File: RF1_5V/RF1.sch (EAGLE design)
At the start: 13 parts, among them J1 5v, Q1 16mhz, U1 ATMEGA328P_PDIP

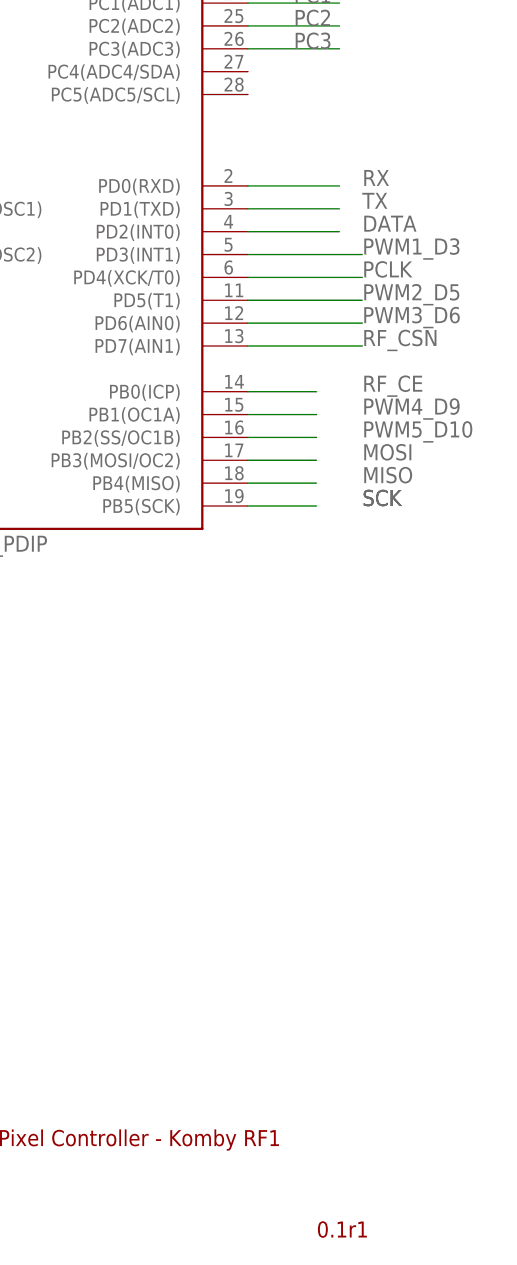
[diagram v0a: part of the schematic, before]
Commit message: Updated with 2014 designs for both RF1_12v and RF1 5v
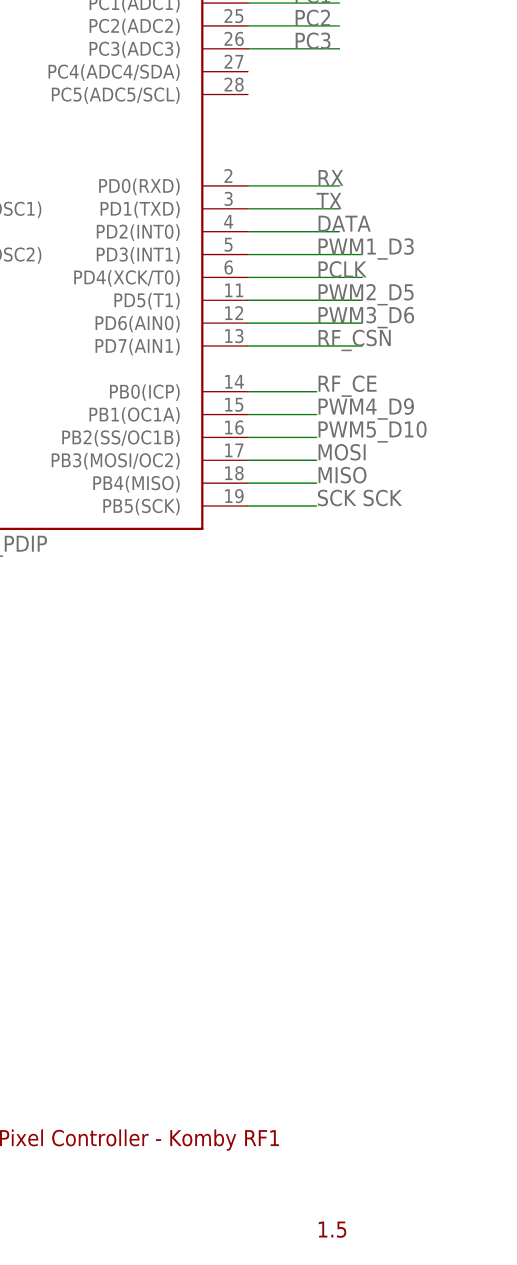
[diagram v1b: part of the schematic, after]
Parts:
- J1: device con-jack:DCJ0303 -> con-jack_komby:DCJ0303
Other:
- note added: "1.5"
- note removed: "0.1r1"
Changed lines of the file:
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@@
 <part name="GND7" library="supply1" deviceset="GND" device=""/>
 <part name="GND9" library="supply1" deviceset="GND" device=""/>
-<part name="J1" library="con-jack" deviceset="DCJ0303" device="" value="5v"/>
+<part name="J1" library="con-jack_komby" deviceset="DCJ0303" device="" value="5v"/>
 <part name="IC1" library="adafruit" deviceset="MCP1700" device="TRI"/>
 <part name="GND1" library="supply1" deviceset="GND" device=""/>
@@
 <plain>
 <text x="172.72" y="17.78" size="1.778" layer="94">Arduino Compatible, Single Pixel Controller - Komby RF1</text>
-<text x="238.76" y="7.62" size="1.778" layer="94">0.1r1</text>
+<text x="238.76" y="7.62" size="1.778" layer="94">1.5</text>
 <text x="154.94" y="7.62" size="1.778" layer="94">http://www.komby.com/RF1</text>
 <text x="38.1" y="15.24" size="1.778" layer="94">This work is licensed under a Creative Commons Attribution-ShareAlike 3.0 United States License.</text>
 </plain>
 <instances>
-<instance part="FRAME1" gate="G$1" x="0" y="0"/>
+<instance part="FRAME1" gate="G$1" x="5.08" y="0"/>
 <instance part="FRAME1" gate="G$2" x="147.32" y="0"/>
 <instance part="U1" gate="G$1" x="205.74" y="121.92"/>
@@
 <net name="SCK" class="0">
 <segment>
-<label x="243.84" y="88.9" size="1.778" layer="95"/>
+<label x="238.76" y="88.9" size="1.778" layer="95"/>
 <label x="243.84" y="88.9" size="1.778" layer="95"/>
 <wire x1="231.14" y1="88.9" x2="238.76" y2="88.9" width="0.1524" layer="91"/>
@@
 <segment>
 <wire x1="231.14" y1="91.44" x2="238.76" y2="91.44" width="0.1524" layer="91"/>
-<label x="243.84" y="91.44" size="1.778" layer="95"/>
+<label x="238.76" y="91.44" size="1.778" layer="95"/>
 <pinref part="U1" gate="G$1" pin="PB4(MISO)"/>
 </segment>
@@
 <segment>
 <wire x1="231.14" y1="93.98" x2="238.76" y2="93.98" width="0.1524" layer="91"/>
-<label x="243.84" y="93.98" size="1.778" layer="95"/>
+<label x="238.76" y="93.98" size="1.778" layer="95"/>
 <pinref part="U1" gate="G$1" pin="PB3(MOSI/OC2)"/>
 </segment>
@@
 <segment>
 <wire x1="231.14" y1="121.92" x2="241.3" y2="121.92" width="0.1524" layer="91"/>
-<label x="243.84" y="121.92" size="1.778" layer="95"/>
+<label x="238.76" y="121.92" size="1.778" layer="95"/>
 <pinref part="U1" gate="G$1" pin="PD1(TXD)"/>
 </segment>
@@
 <segment>
 <wire x1="231.14" y1="124.46" x2="241.3" y2="124.46" width="0.1524" layer="91"/>
-<label x="243.84" y="124.46" size="1.778" layer="95"/>
+<label x="238.76" y="124.46" size="1.778" layer="95"/>
 <pinref part="U1" gate="G$1" pin="PD0(RXD)"/>
 </segment>
@@
 <segment>
 <wire x1="231.14" y1="119.38" x2="241.3" y2="119.38" width="0.1524" layer="91"/>
-<label x="243.84" y="119.38" size="1.778" layer="95"/>
+<label x="238.76" y="119.38" size="1.778" layer="95"/>
 <pinref part="U1" gate="G$1" pin="PD2(INT0)"/>
 </segment>
@@
 <segment>
 <wire x1="231.14" y1="114.3" x2="243.84" y2="114.3" width="0.1524" layer="91"/>
-<label x="243.84" y="114.3" size="1.778" layer="95"/>
+<label x="238.76" y="114.3" size="1.778" layer="95"/>
 <pinref part="U1" gate="G$1" pin="PD4(XCK/T0)"/>
 </segment>
@@
 <segment>
 <wire x1="231.14" y1="111.76" x2="243.84" y2="111.76" width="0.1524" layer="91"/>
-<label x="243.84" y="111.76" size="1.778" layer="95"/>
+<label x="238.76" y="111.76" size="1.778" layer="95"/>
 <pinref part="U1" gate="G$1" pin="PD5(T1)"/>
 </segment>
@@
 <segment>
 <wire x1="231.14" y1="96.52" x2="238.76" y2="96.52" width="0.1524" layer="91"/>
-<label x="243.84" y="96.52" size="1.778" layer="95"/>
+<label x="238.76" y="96.52" size="1.778" layer="95"/>
 <pinref part="U1" gate="G$1" pin="PB2(SS/OC1B)"/>
 </segment>
@@
 </segment>
 <segment>
-<label x="243.84" y="99.06" size="1.778" layer="95"/>
+<label x="238.76" y="99.06" size="1.778" layer="95"/>
 <wire x1="231.14" y1="99.06" x2="238.76" y2="99.06" width="0.1524" layer="91"/>
 <pinref part="U1" gate="G$1" pin="PB1(OC1A)"/>
@@
 <pinref part="U1" gate="G$1" pin="PD6(AIN0)"/>
 <wire x1="231.14" y1="109.22" x2="243.84" y2="109.22" width="0.1524" layer="91"/>
-<label x="243.84" y="109.22" size="1.778" layer="95"/>
+<label x="238.76" y="109.22" size="1.778" layer="95"/>
 </segment>
 </net>
@@
 <segment>
 <wire x1="231.14" y1="116.84" x2="243.84" y2="116.84" width="0.1524" layer="91"/>
-<label x="243.84" y="116.84" size="1.778" layer="95"/>
+<label x="238.76" y="116.84" size="1.778" layer="95"/>
 <pinref part="U1" gate="G$1" pin="PD3(INT1)"/>
 </segment>
@@
 <segment>
 <wire x1="231.14" y1="106.68" x2="243.84" y2="106.68" width="0.1524" layer="91"/>
-<label x="243.84" y="106.68" size="1.778" layer="95"/>
+<label x="238.76" y="106.68" size="1.778" layer="95"/>
 <pinref part="U1" gate="G$1" pin="PD7(AIN1)"/>
 </segment>
@@
 <segment>
 <wire x1="231.14" y1="101.6" x2="238.76" y2="101.6" width="0.1524" layer="91"/>
-<label x="243.84" y="101.6" size="1.778" layer="95"/>
+<label x="238.76" y="101.6" size="1.778" layer="95"/>
 <pinref part="U1" gate="G$1" pin="PB0(ICP)"/>
 </segment>
